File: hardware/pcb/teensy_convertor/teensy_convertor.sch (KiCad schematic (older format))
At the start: 5 parts, among them J101 CONN_01X03, U1 Teensy-3.2, U101 MicroC_Header

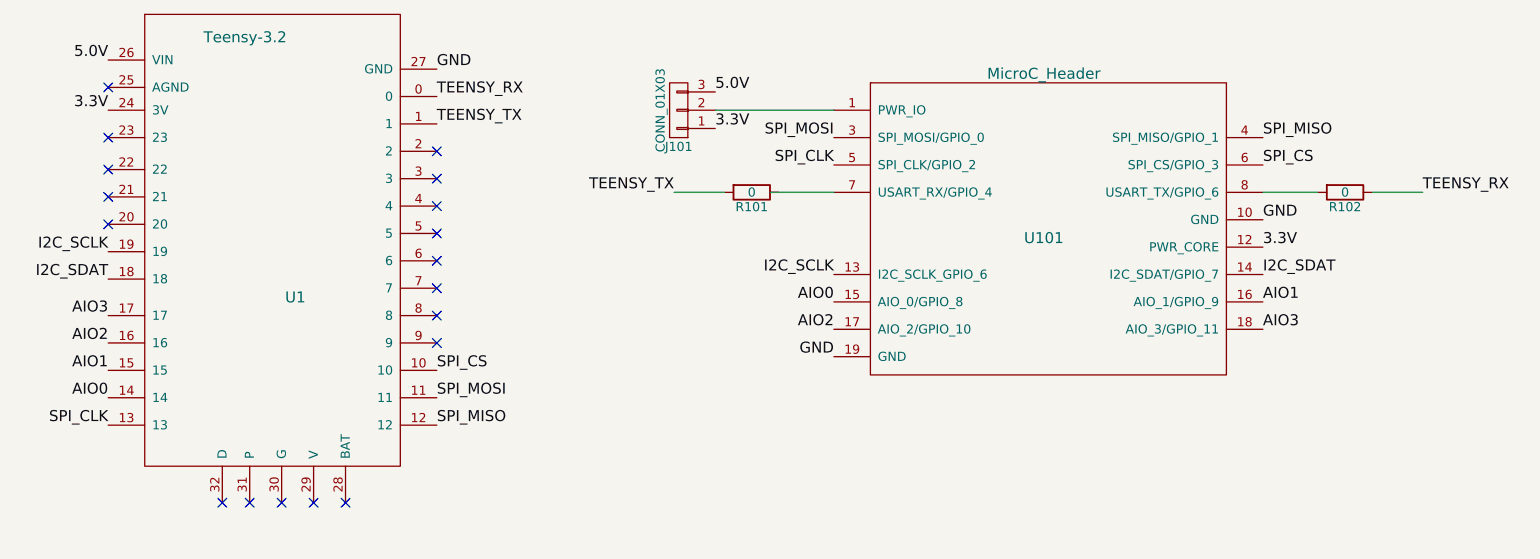
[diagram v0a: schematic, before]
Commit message: Initial layout
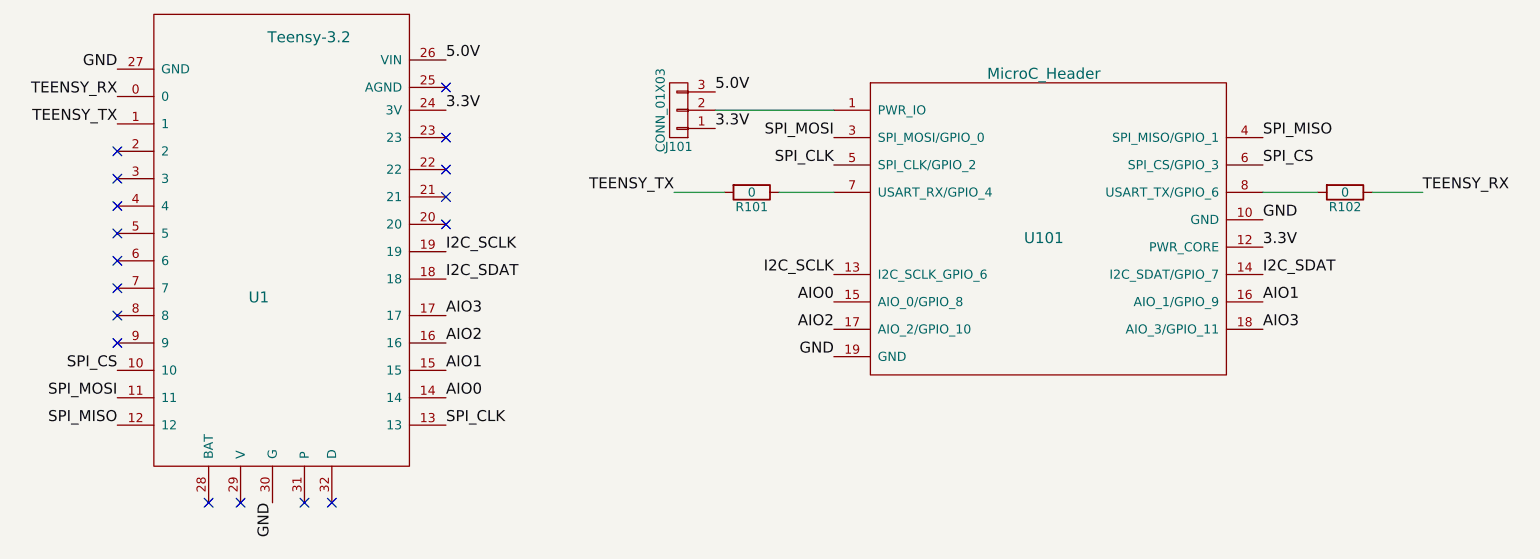
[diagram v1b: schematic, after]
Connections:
- no-connect marks 18 -> 17
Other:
- moved on the sheet: U1
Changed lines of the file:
@@
 L Teensy-3.2 U1
 U 1 1 586B0354
-P 3000 3625
-F 0 "U1" H 3150 3375 60  0000 C CNN
-F 1 "Teensy-3.2" H 2875 4800 60  0000 C CNN
-F 2 "teensy_convertor:Teensy-32" H 2775 3300 60  0001 C CNN
-F 3 "" H 2775 3300 60  0001 C CNN
-	1    3000 3625
-	1    0    0    -1
+P 3100 3625
+F 0 "U1" H 3250 3375 60  0000 C CNN
+F 1 "Teensy-3.2" H 2975 4800 60  0000 C CNN
+F 2 "teensy_convertor:Teensy-32" H 2875 3300 60  0001 C CNN
+F 3 "" H 2875 3300 60  0001 C CNN
+	1    3100 3625
+	-1   0    0    -1
 $EndComp
 $Comp
@@
 	-1   0    0    1
 $EndComp
-Text Label 2125 2850 2    60   ~ 0
+Text Label 3975 2850 0    60   ~ 0
 3.3V
 Text Label 5450 2950 0    60   ~ 0
@@
 Text Label 8450 3600 0    60   ~ 0
 3.3V
-Text Label 2125 2575 2    60   ~ 0
+Text Label 3975 2575 0    60   ~ 0
 5.0V
 Text Label 5450 2750 0    60   ~ 0
@@
 Text Label 6100 4200 2    60   ~ 0
 GND
-Text Label 3925 2625 0    60   ~ 0
+Text Label 2175 2625 2    60   ~ 0
 GND
 Text Label 6100 3000 2    60   ~ 0
 SPI_MOSI
-Text Label 3925 4425 0    60   ~ 0
+Text Label 2175 4425 2    60   ~ 0
 SPI_MOSI
 Text Label 6100 3150 2    60   ~ 0
 SPI_CLK
-Text Label 2125 4575 2    60   ~ 0
+Text Label 3975 4575 0    60   ~ 0
 SPI_CLK
 Text Label 8450 3000 0    60   ~ 0
 SPI_MISO
-Text Label 3925 4575 0    60   ~ 0
+Text Label 2175 4575 2    60   ~ 0
 SPI_MISO
 Text Label 8450 3150 0    60   ~ 0
 SPI_CS
-Text Label 3925 4275 0    60   ~ 0
+Text Label 2175 4275 2    60   ~ 0
 SPI_CS
 $Comp
@@
 	6100 2850 5450 2850
 Wire Wire Line
-	5750 3300 6100 3300
+	5800 3300 6100 3300
 Wire Wire Line
 	8450 3300 8750 3300
@@
 Text Label 9325 3300 0    60   ~ 0
 TEENSY_RX
-Text Label 3925 2775 0    60   ~ 0
+Text Label 2175 2775 2    60   ~ 0
 TEENSY_RX
 Text Label 5225 3300 2    60   ~ 0
 TEENSY_TX
-Text Label 3925 2925 0    60   ~ 0
+Text Label 2175 2925 2    60   ~ 0
 TEENSY_TX
 Text Label 6100 3750 2    60   ~ 0
 I2C_SCLK
-Text Label 2125 3625 2    60   ~ 0
+Text Label 3975 3625 0    60   ~ 0
 I2C_SCLK
-Text Label 2125 3775 2    60   ~ 0
+Text Label 3975 3775 0    60   ~ 0
 I2C_SDAT
 Text Label 8450 3750 0    60   ~ 0
@@
 Text Label 6100 3900 2    60   ~ 0
 AIO0
-Text Label 2125 4425 2    60   ~ 0
+Text Label 3975 4425 0    60   ~ 0
 AIO0
 Text Label 6100 4050 2    60   ~ 0
@@
 Text Label 8450 4050 0    60   ~ 0
 AIO3
-Text Label 2125 4125 2    60   ~ 0
+Text Label 3975 4125 0    60   ~ 0
 AIO2
-Text Label 2125 4275 2    60   ~ 0
+Text Label 3975 4275 0    60   ~ 0
 AIO1
-Text Label 2125 3975 2    60   ~ 0
+Text Label 3975 3975 0    60   ~ 0
 AIO3
-NoConn ~ 3925 3075
-NoConn ~ 3925 3225
-NoConn ~ 3925 3375
-NoConn ~ 3925 3525
-NoConn ~ 3925 3675
-NoConn ~ 3925 3825
-NoConn ~ 3925 3975
-NoConn ~ 3925 4125
-NoConn ~ 3425 5000
-NoConn ~ 3250 5000
-NoConn ~ 3075 5000
-NoConn ~ 2900 5000
-NoConn ~ 2750 5000
-NoConn ~ 2125 3475
-NoConn ~ 2125 3325
-NoConn ~ 2125 3175
-NoConn ~ 2125 3000
-NoConn ~ 2125 2725
+NoConn ~ 2175 3075
+NoConn ~ 2175 3225
+NoConn ~ 2175 3375
+NoConn ~ 2175 3525
+NoConn ~ 2175 3675
+NoConn ~ 2175 3825
+NoConn ~ 2175 3975
+NoConn ~ 2175 4125
+NoConn ~ 2675 5000
+NoConn ~ 2850 5000
+NoConn ~ 3200 5000
+NoConn ~ 3350 5000
+NoConn ~ 3975 3475
+NoConn ~ 3975 3325
+NoConn ~ 3975 3175
+NoConn ~ 3975 3000
+NoConn ~ 3975 2725
+Text Label 3025 5000 3    60   ~ 0
+GND
 $EndSCHEMATC
